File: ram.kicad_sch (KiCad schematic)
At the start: 42 parts, among them IC11 HM514260AJ8, IC25 74LVC139, IC6 HM514260AJ8, U2 TXS0108EPW, U3 TXS0108EPW, U4 TXS0108EPW, U5 TXS0108EPW, U6 IS41LV16105D, U7 IS41LV16105D, U8 TXS0108EPW, U9 TXS0108EPW

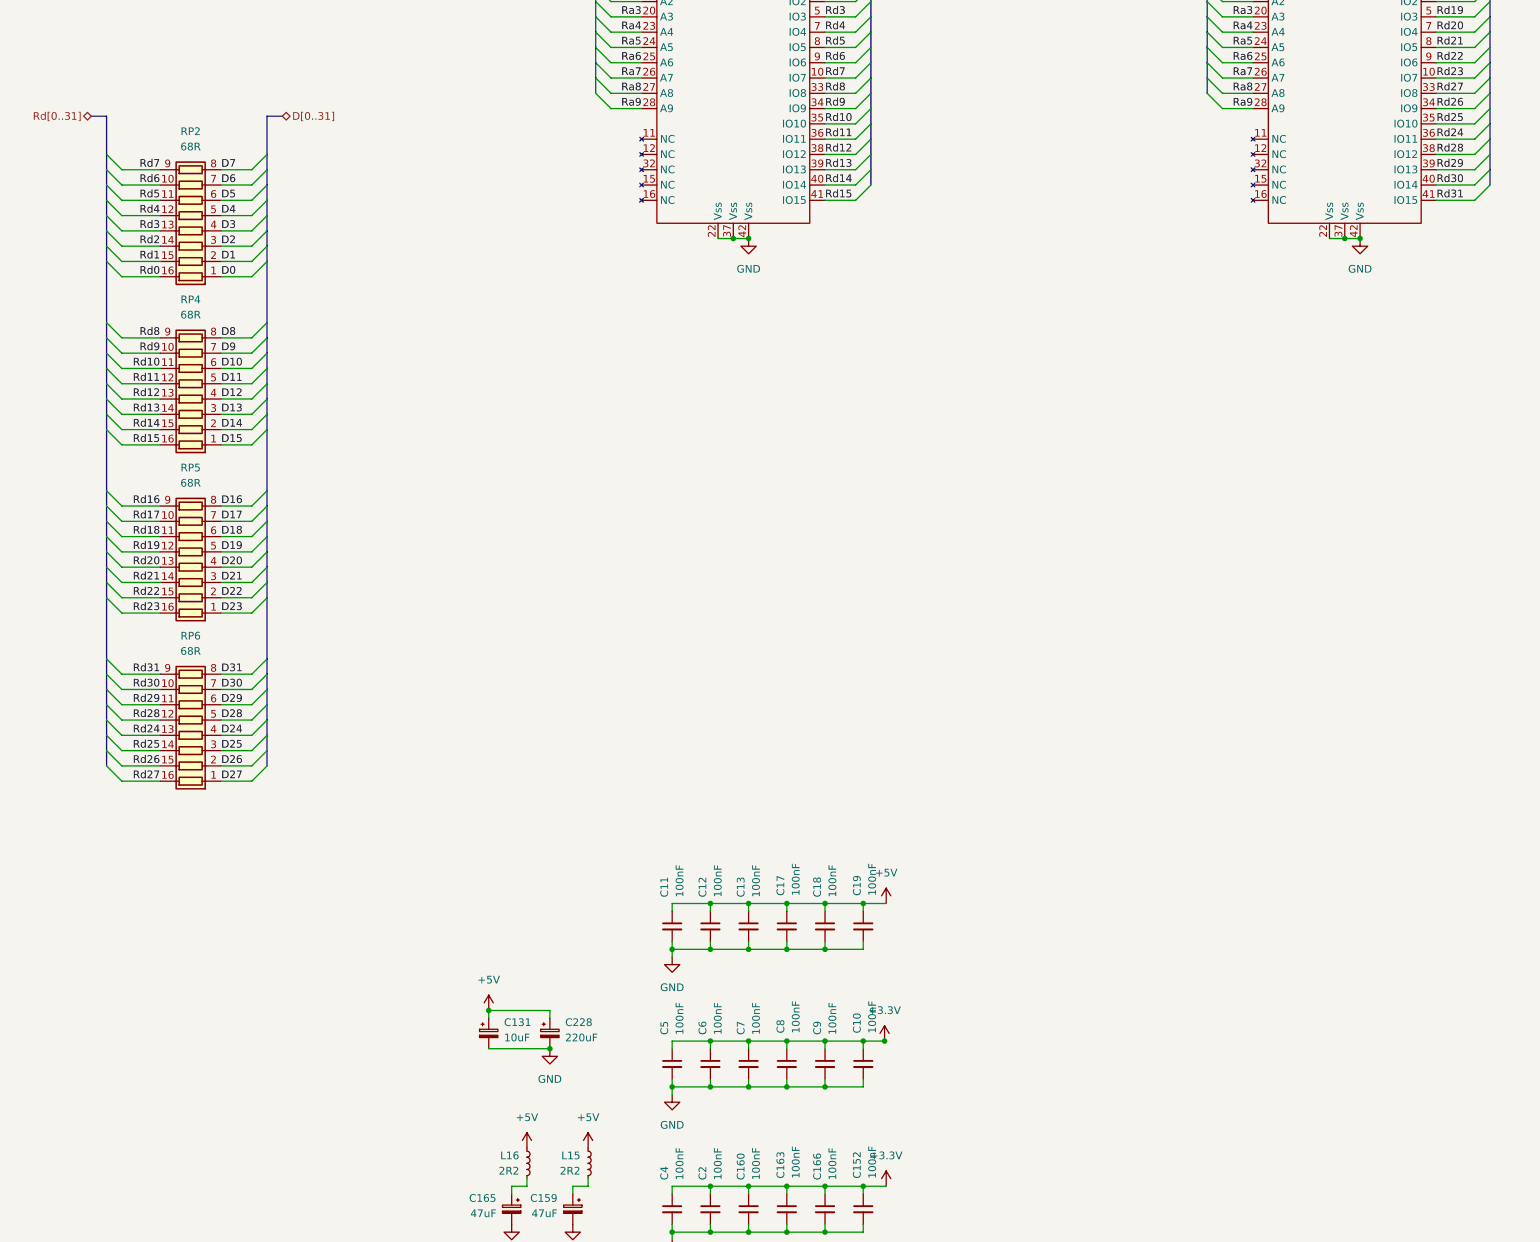
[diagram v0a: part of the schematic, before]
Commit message: prepare for fabrication
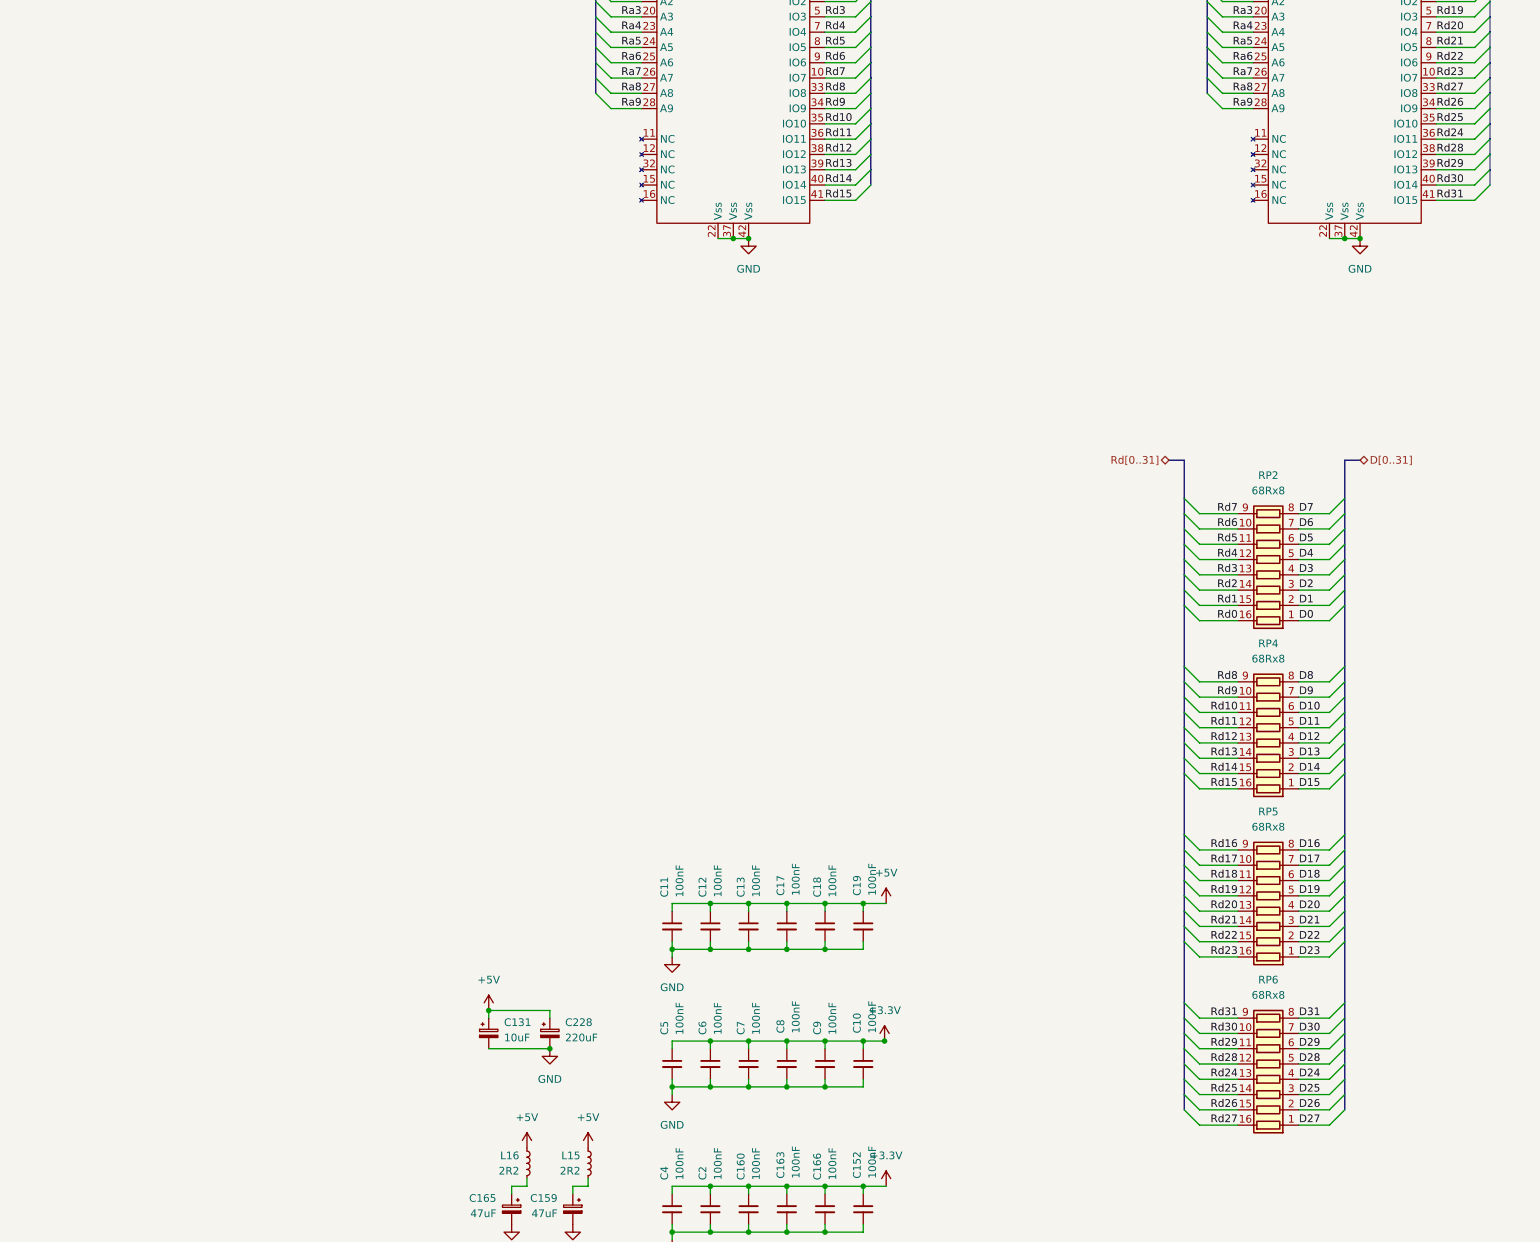
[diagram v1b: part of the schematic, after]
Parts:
- C10, C11, C12, C13, C152, C160, C162, C163, C166, C17, C18, C19, C2, C4, C5, C6, C7, C8, C9: LCSC (none) -> C49678; LCSC Part (none) -> C49678
- IC25: LCSC (none) -> C7662; LCSC Part (none) -> C7662
- R135: LCSC (none) -> C17630; LCSC Part (none) -> C17630
- R136: LCSC (none) -> C2907219; LCSC Part (none) -> C2907219
- RP2, RP4, RP5, RP6: value 68R -> 68Rx8; LCSC (none) -> C1739978; LCSC Part (none) -> C1739978
- U2, U3, U4, U5, U8, U9: LCSC (none) -> C17206; LCSC Part (none) -> C17206
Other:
- moved on the sheet: RP2, RP4, RP5, RP6
